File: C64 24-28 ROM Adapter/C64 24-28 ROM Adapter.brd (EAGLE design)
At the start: 38.1 x 21.3 mm, 2 parts

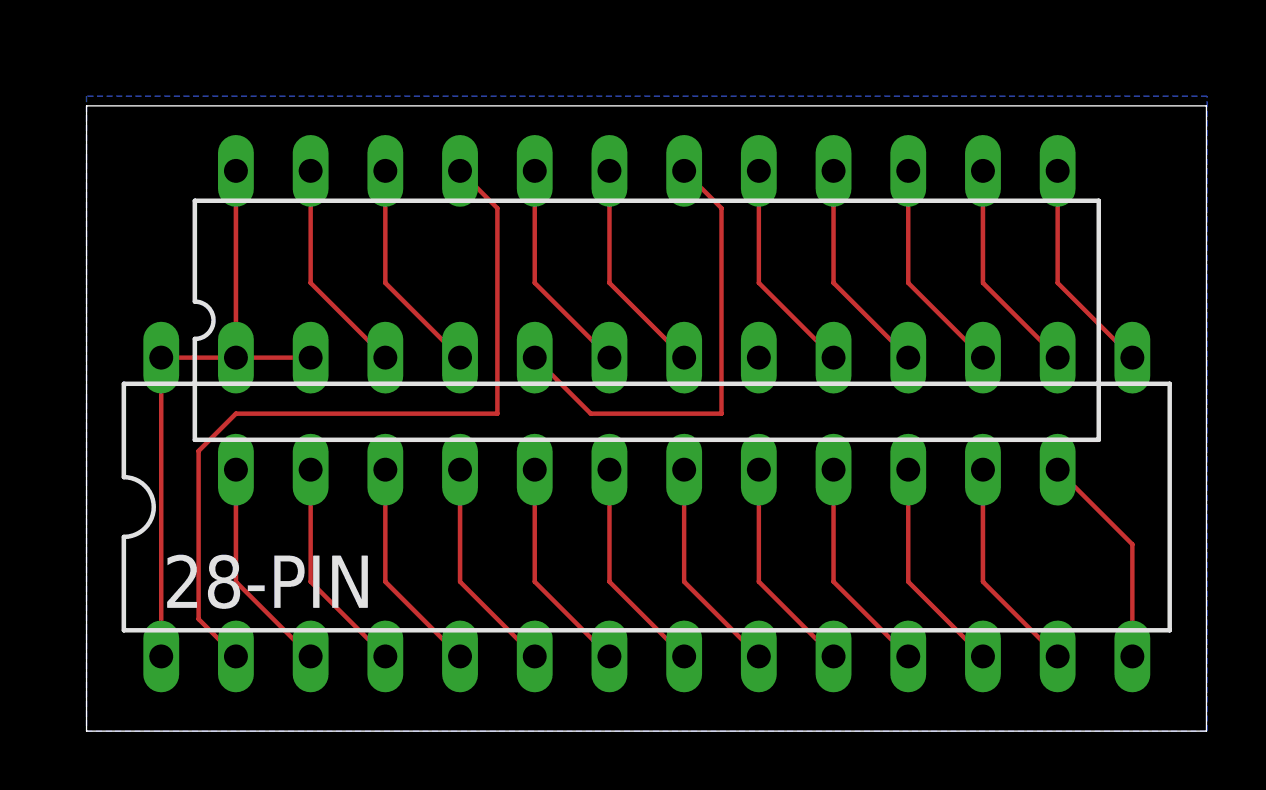
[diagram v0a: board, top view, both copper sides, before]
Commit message: Update Commit
Haven't commited in forever, sending an update!
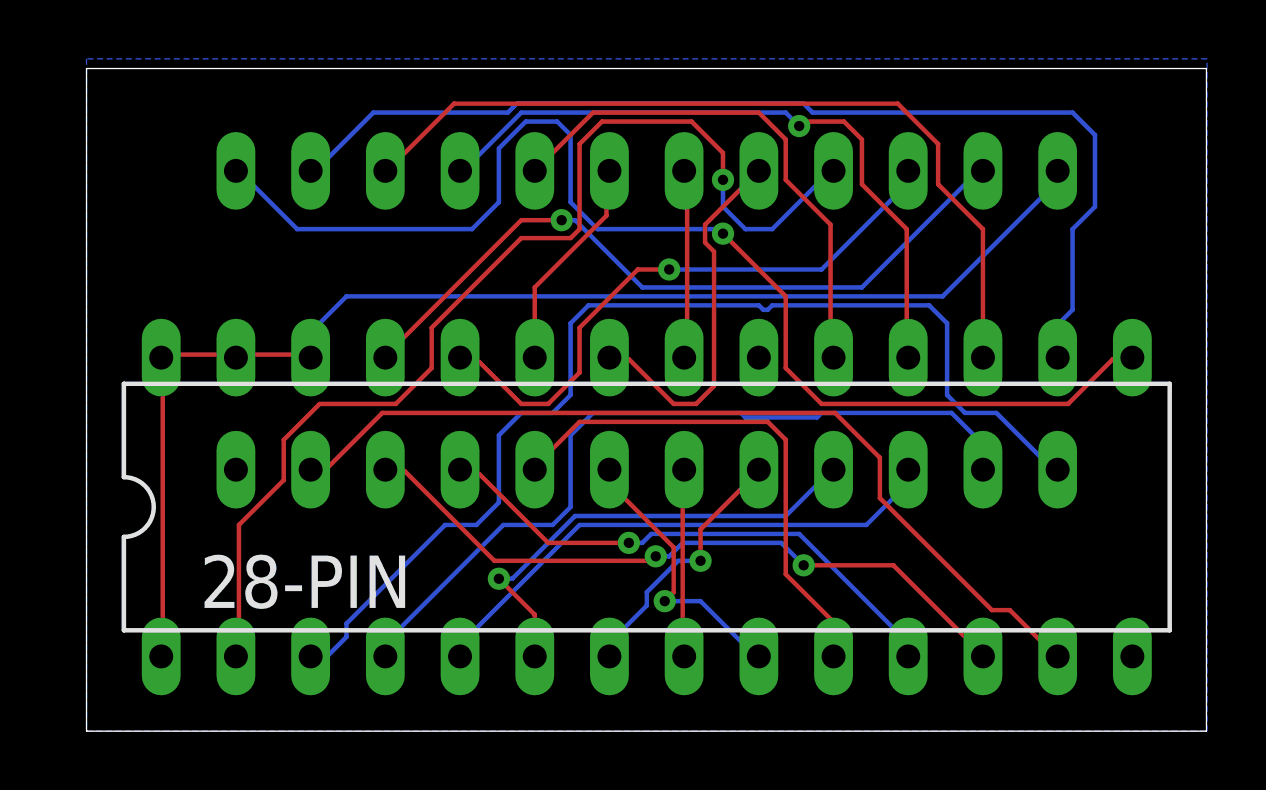
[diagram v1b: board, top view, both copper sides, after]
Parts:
- flipped 24-PIN to the bottom
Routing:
- net D3: track 7.40 -> 41.3 mm, vias 0 -> 1
- net A7: track 7.40 -> 37.3 mm
- net D4: track 7.40 -> 36.1 mm
- net D2: track 7.40 -> 30.5 mm
- net VCC: track 21.6 -> 44.4 mm
- net D5: track 7.40 -> 28.2 mm
- net A6: track 7.40 -> 26.9 mm
- net A8: track 7.40 -> 24.9 mm, vias 0 -> 1
- net D1: track 7.40 -> 23.5 mm, vias 0 -> 2
- net D6: track 7.40 -> 23.1 mm, vias 0 -> 1
- net A9: track 7.40 -> 20.3 mm, vias 0 -> 1
- net A5: track 7.40 -> 18.4 mm
- net D0: track 7.40 -> 18.4 mm, vias 0 -> 1
- net D7: track 7.40 -> 17.8 mm
- net A0: track 7.40 -> 17.6 mm
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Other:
- board size 38.1 x 21.3 mm -> 38.1 x 22.5 mm
- board text added: "24-PIN"
